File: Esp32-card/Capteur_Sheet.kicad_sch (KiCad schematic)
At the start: 7 parts, among them J2 Conn_01x02_Pin, J3 Conn_01x02_Pin, J4 Conn_01x03_Pin, J5 Conn_01x03_Pin, J6 Conn_01x03_Pin

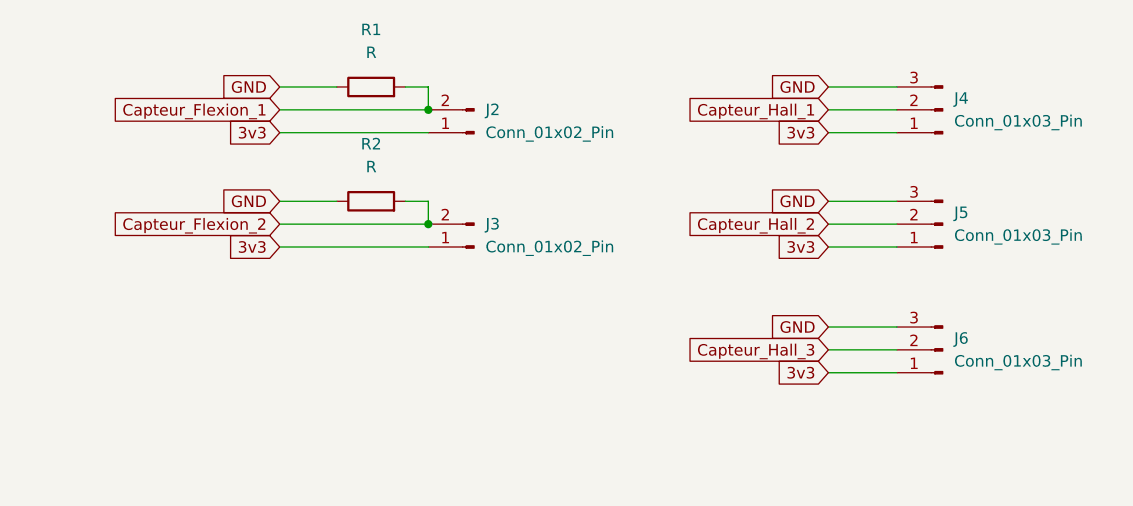
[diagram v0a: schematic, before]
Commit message: .
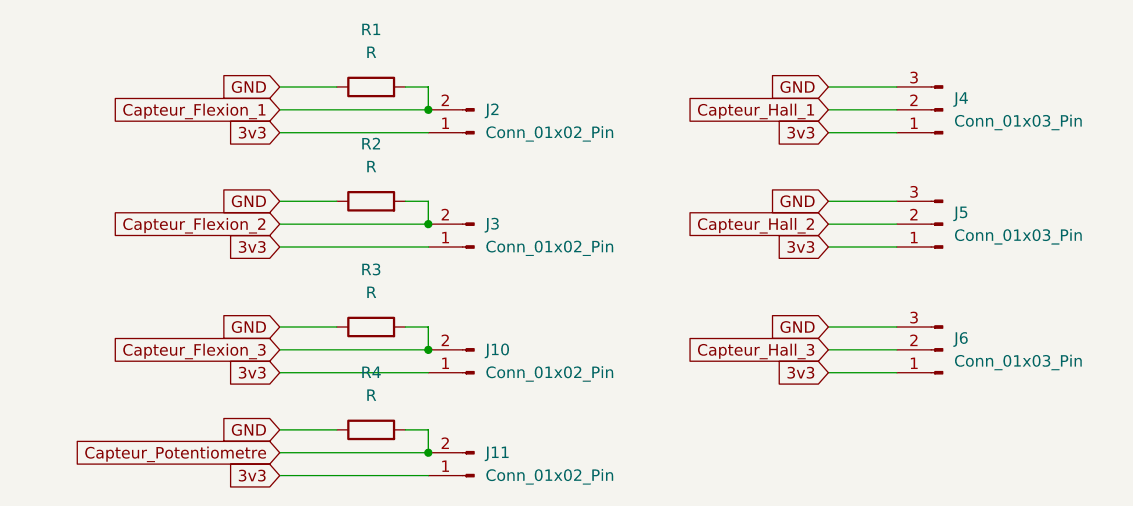
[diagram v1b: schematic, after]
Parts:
- added J10, J11: Conn_01x02_Pin, Connector_PinHeader_2.54mm:PinHeader_1x02_P2.54mm_Horizontal, symbol Connector:Conn_01x02_Pin
- added R3, R4: R, Resistor_THT:R_Axial_DIN0207_L6.3mm_D2.5mm_P7.62mm_Horizontal, symbol Device:R
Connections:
- net 3v3: now also J10.1 (Pin_1), J11.1 (Pin_1)
- net GND: now also R3.1, R4.1
- new net Capteur_Flexion_3: J10.2 (Pin_2), R3.2
- new net Capteur_Potentiometre: J11.2 (Pin_2), R4.2
